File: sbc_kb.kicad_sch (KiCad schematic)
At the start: 18 parts, among them J1 Mini-DIN-6, J2 Mini-DIN-6, U4 7406, U9 VT82C42 PS2 CONTROLLER

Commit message: minor BOM tweaks due part availability. make some pcb routing a little nicer.
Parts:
- F1: LCSC Part # C3760254 -> C2687078
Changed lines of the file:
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@@
 			)
 		)
-		(property "Description" "LCSC #C3760254"
+		(property "Description" "LCSC #C3760254 (Bourns) or LCSC #C2687078"
 			(at 60.96 30.48 0)
 			(effects
@@
 			)
 		)
-		(property "LCSC Part #" "C3760254"
+		(property "LCSC Part #" "C2687078"
 			(at 60.96 30.48 0)
 			(effects

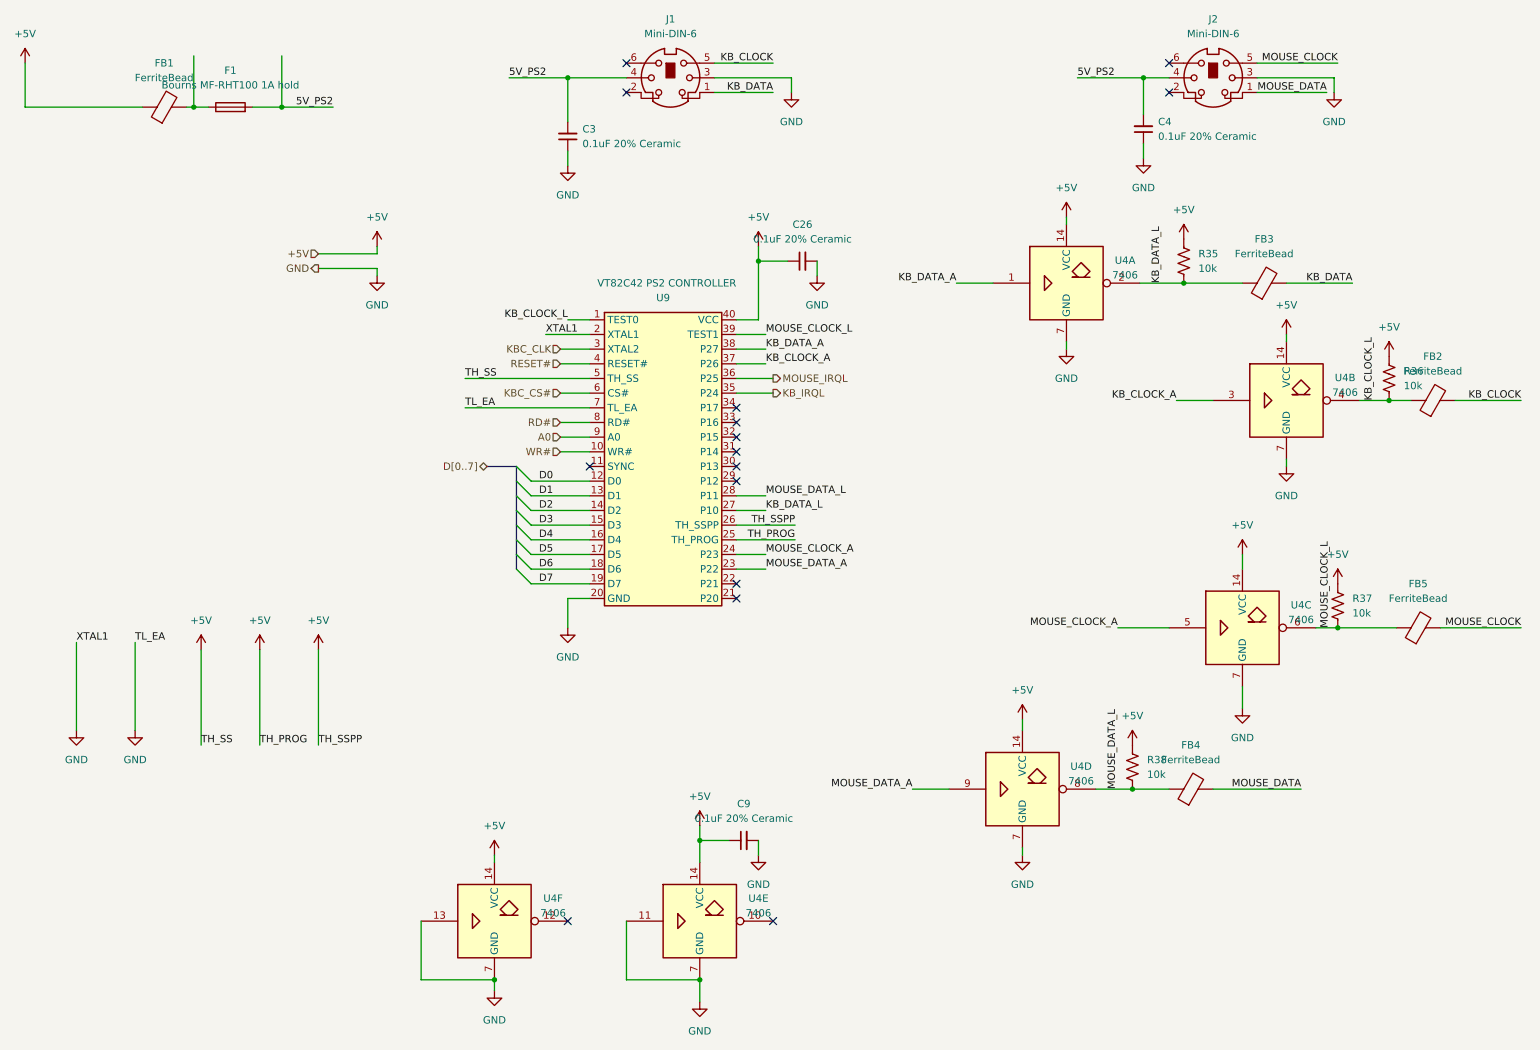
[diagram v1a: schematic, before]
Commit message: no more SMT for isa_i2c, tweak motherboard multiplex logic, handful of other tweaks
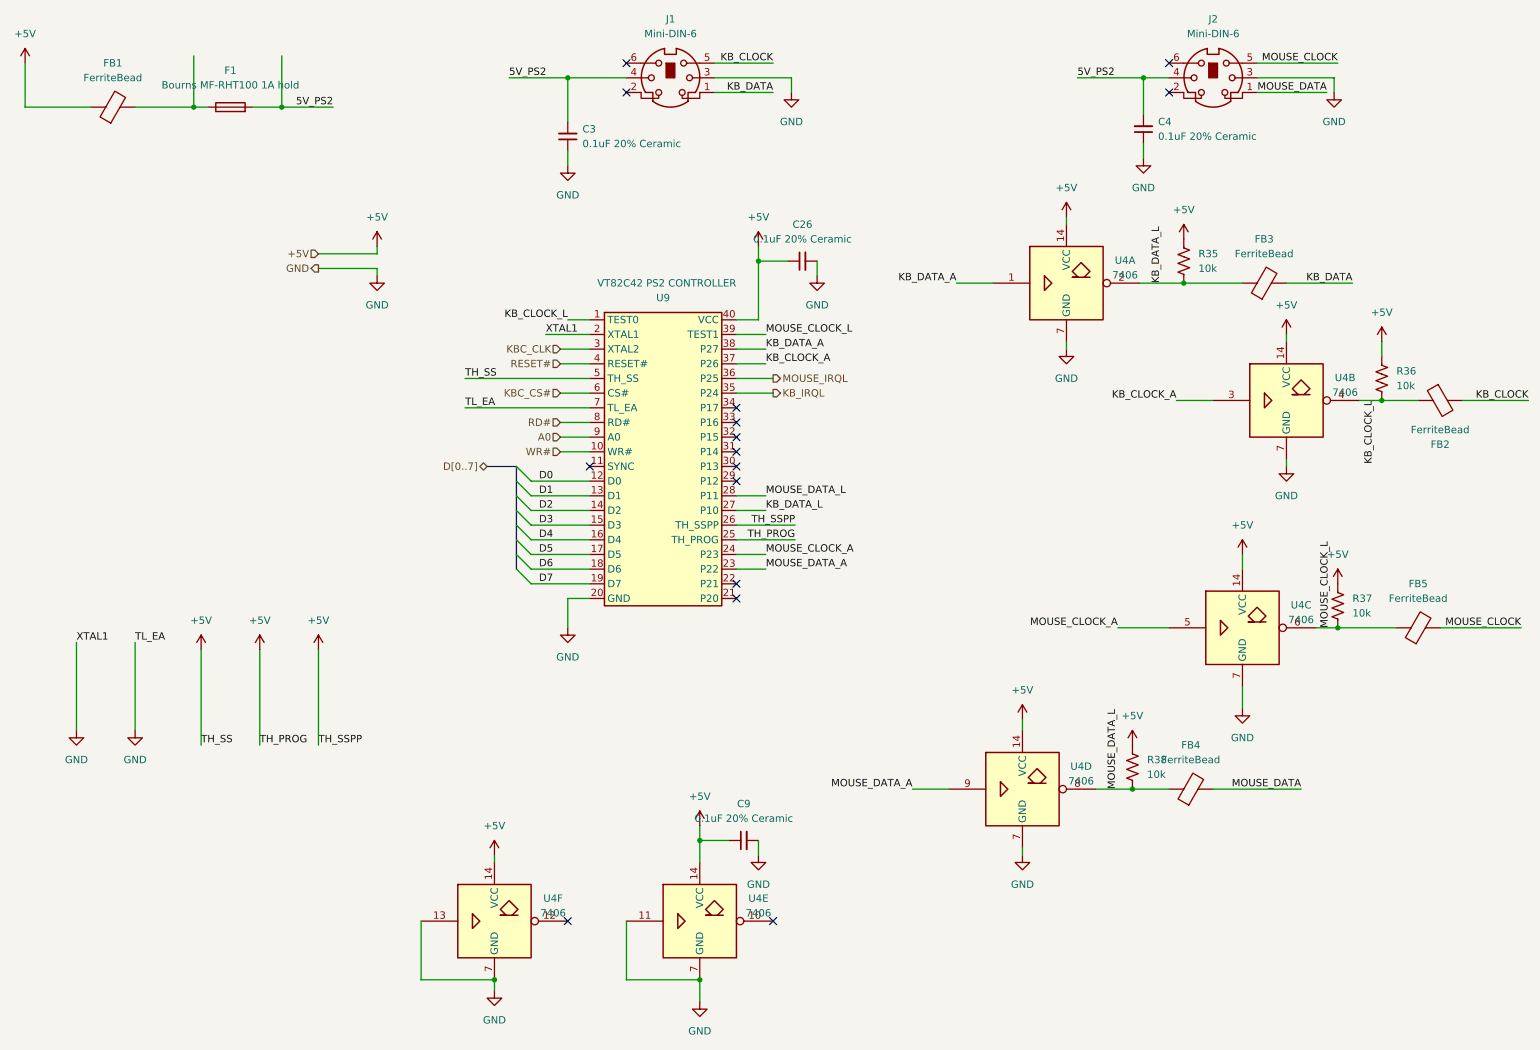
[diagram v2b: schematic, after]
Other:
- moved on the sheet: FB1, FB2, R36
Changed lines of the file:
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@@
 	)
 	(junction
+		(at 260.35 81.28)
+		(diameter 0)
+		(color 0 0 0 0)
+	)
+	(junction
 		(at 119.38 25.4)
 		(diameter 0)
@@
 		(color 0 0 0 0)
 	)
-	(junction
-		(at 261.62 81.28)
-		(diameter 0)
-		(color 0 0 0 0)
-	)
 	(no_connect
 		(at 129.54 27.94)
@@
 	(wire
 		(pts
-			(xy 25.4 30.48) (xy 45.72 30.48)
+			(xy 25.4 30.48) (xy 36.83 30.48)
 		)
 		(stroke
@@
 	(wire
 		(pts
-			(xy 53.34 30.48) (xy 54.61 30.48)
-		)
-		(stroke
-			(width 0)
-			(type default)
-		)
-	)
-	(wire
-		(pts
-			(xy 261.62 81.28) (xy 265.43 81.28)
+			(xy 44.45 30.48) (xy 54.61 30.48)
 		)
 		(stroke
@@
 	(wire
 		(pts
+			(xy 260.35 81.28) (xy 266.7 81.28)
+		)
+		(stroke
+			(width 0)
+			(type default)
+		)
+	)
+	(wire
+		(pts
 			(xy 231.14 148.59) (xy 246.38 148.59)
 		)
@@
 	(wire
 		(pts
-			(xy 256.54 81.28) (xy 261.62 81.28)
+			(xy 256.54 81.28) (xy 260.35 81.28)
 		)
 		(stroke
@@
 	(wire
 		(pts
+			(xy 260.35 73.66) (xy 260.35 71.12)
+		)
+		(stroke
+			(width 0)
+			(type default)
+		)
+	)
+	(wire
+		(pts
 			(xy 238.76 25.4) (xy 252.095 25.4)
 		)
@@
 	(wire
 		(pts
-			(xy 273.05 81.28) (xy 284.48 81.28)
+			(xy 274.32 81.28) (xy 285.75 81.28)
 		)
 		(stroke
@@
 	)
 	(label "KB_CLOCK"
-		(at 284.48 81.28 180)
+		(at 285.75 81.28 180)
 		(fields_autoplaced yes)
 		(effects
@@
 	)
 	(label "KB_CLOCK_L"
-		(at 259.08 81.28 90)
+		(at 259.08 81.28 270)
 		(fields_autoplaced yes)
 		(effects
@@
 				(size 1.27 1.27)
 			)
-			(justify left bottom)
+			(justify right bottom)
 		)
 	)
@@
 	(symbol
 		(lib_id "Device:FerriteBead")
-		(at 49.53 30.48 90)
+		(at 40.64 30.48 90)
 		(unit 1)
 		(exclude_from_sim no)
@@
 		(fields_autoplaced yes)
 		(property "Reference" "FB1"
-			(at 49.4792 22.86 90)
+			(at 40.5892 22.86 90)
 			(effects
 				(font
@@
 		)
 		(property "Value" "FerriteBead"
-			(at 49.4792 25.4 90)
+			(at 40.5892 25.4 90)
 			(effects
 				(font
@@
 		)
 		(property "Footprint" "Inductor_SMD:L_1206_3216Metric"
-			(at 49.53 32.258 90)
+			(at 40.64 32.258 90)
 			(effects
 				(font
@@
 		)
 		(property "Datasheet" "~"
-			(at 49.53 30.48 0)
+			(at 40.64 30.48 0)
 			(effects
 				(font
@@
 		)
 		(property "Description" "LCSC #C92887"
-			(at 49.53 30.48 0)
+			(at 40.64 30.48 0)
 			(effects
 				(font
@@
 		)
 		(property "Height" ""
-			(at 49.53 30.48 0)
+			(at 40.64 30.48 0)
 			(effects
 				(font
@@
 		)
 		(property "Manufacturer_Name" ""
-			(at 49.53 30.48 0)
+			(at 40.64 30.48 0)
 			(effects
 				(font
@@
 		)
 		(property "Manufacturer_Part_Number" ""
-			(at 49.53 30.48 0)
+			(at 40.64 30.48 0)
 			(effects
 				(font
@@
 		)
 		(property "Mouser Part Number" ""
-			(at 49.53 30.48 0)
+			(at 40.64 30.48 0)
 			(effects
 				(font
@@
 		)
 		(property "Mouser Price/Stock" ""
-			(at 49.53 30.48 0)
+			(at 40.64 30.48 0)
 			(effects
 				(font
@@
 		)
 		(property "LCSC Part #" "C92887"
-			(at 49.53 30.48 0)
+			(at 40.64 30.48 0)
 			(effects
 				(font
@@
 	(symbol
 		(lib_id "Device:R_US")
-		(at 261.62 77.47 0)
+		(at 260.35 77.47 0)
 		(unit 1)
 		(exclude_from_sim no)
@@
 		(fields_autoplaced yes)
 		(property "Reference" "R36"
-			(at 264.16 76.2 0)
+			(at 262.89 76.2 0)
 			(effects
 				(font
@@
 		)
 		(property "Value" "10k"
-			(at 264.16 78.74 0)
+			(at 262.89 78.74 0)
 			(effects
 				(font
@@
 		)
 		(property "Footprint" "Resistor_SMD:R_0805_2012Metric"
-			(at 262.636 77.724 90)
+			(at 261.366 77.724 90)
 			(effects
 				(font
@@
 		)
 		(property "Datasheet" "~"
-			(at 261.62 77.47 0)
+			(at 260.35 77.47 0)
 			(effects
 				(font
@@
 		)
 		(property "Description" "LCSC #C84376 "
-			(at 261.62 77.47 0)
+			(at 260.35 77.47 0)
 			(effects
 				(font
@@
 		)
 		(property "Height" ""
-			(at 261.62 77.47 0)
+			(at 260.35 77.47 0)
 			(effects
 				(font
@@
 		)
 		(property "Manufacturer_Name" ""
-			(at 261.62 77.47 0)
+			(at 260.35 77.47 0)
 			(effects
 				(font
@@
 		)
 		(property "Manufacturer_Part_Number" ""
-			(at 261.62 77.47 0)
+			(at 260.35 77.47 0)
 			(effects
 				(font
@@
 		)
 		(property "Mouser Part Number" ""
-			(at 261.62 77.47 0)
+			(at 260.35 77.47 0)
 			(effects
 				(font
@@
 		)
 		(property "Mouser Price/Stock" ""
-			(at 261.62 77.47 0)
+			(at 260.35 77.47 0)
 			(effects
 				(font
@@
 		)
 		(property "LCSC Part #" "C84376 "
-			(at 261.62 77.47 0)
+			(at 260.35 77.47 0)
 			(effects
 				(font
@@
 	(symbol
 		(lib_id "Device:FerriteBead")
-		(at 269.24 81.28 90)
+		(at 270.51 81.28 90)
+		(mirror x)
 		(unit 1)
 		(exclude_from_sim no)
@@
 		(dnp no)
 		(property "Reference" "FB2"
-			(at 269.1892 73.66 90)
+			(at 270.4592 88.9 90)
 			(effects
 				(font
@@
 		)
 		(property "Value" "FerriteBead"
-			(at 269.1892 76.2 90)
+			(at 270.4592 86.36 90)
 			(effects
 				(font
@@
 		)
 		(property "Footprint" "Inductor_SMD:L_1206_3216Metric"
-			(at 269.24 83.058 90)
+			(at 270.51 79.502 90)
 			(effects
 				(font
@@
 		)
 		(property "Datasheet" "~"
-			(at 269.24 81.28 0)
+			(at 270.51 81.28 0)
 			(effects
 				(font
@@
 		)
 		(property "Description" "LCSC #C92887"
-			(at 269.24 81.28 0)
+			(at 270.51 81.28 0)
 			(effects
 				(font
@@
 		)
 		(property "Height" ""
-			(at 269.24 81.28 0)
+			(at 270.51 81.28 0)
 			(effects
 				(font
@@
 		)
 		(property "Manufacturer_Name" ""
-			(at 269.24 81.28 0)
+			(at 270.51 81.28 0)
 			(effects
 				(font
@@
 		)
 		(property "Manufacturer_Part_Number" ""
-			(at 269.24 81.28 0)
+			(at 270.51 81.28 0)
 			(effects
 				(font
@@
 		)
 		(property "Mouser Part Number" ""
-			(at 269.24 81.28 0)
+			(at 270.51 81.28 0)
 			(effects
 				(font
@@
 		)
 		(property "Mouser Price/Stock" ""
-			(at 269.24 81.28 0)
+			(at 270.51 81.28 0)
 			(effects
 				(font
@@
 		)
 		(property "LCSC Part #" "C92887"
-			(at 269.24 81.28 0)
+			(at 270.51 81.28 0)
 			(effects
 				(font
@@
 	(symbol
 		(lib_id "power:+5V")
-		(at 261.62 73.66 0)
+		(at 260.35 71.12 0)
 		(unit 1)
 		(exclude_from_sim no)
@@
 		(fields_autoplaced yes)
 		(property "Reference" "#PWR0314"
-			(at 261.62 77.47 0)
+			(at 260.35 74.93 0)
 			(effects
 				(font
@@
 		)
 		(property "Value" "+5V"
-			(at 261.62 68.58 0)
+			(at 260.35 66.04 0)
 			(effects
 				(font
@@
 		)
 		(property "Footprint" ""
-			(at 261.62 73.66 0)
+			(at 260.35 71.12 0)
 			(effects
 				(font
@@
 		)
 		(property "Datasheet" ""
-			(at 261.62 73.66 0)
+			(at 260.35 71.12 0)
 			(effects
 				(font
@@
 		)
 		(property "Description" ""
-			(at 261.62 73.66 0)
+			(at 260.35 71.12 0)
 			(effects
 				(font

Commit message: motherboard tweaks for manufacturing run, i2c card tweaks for manufacturing run, de9 -> stemma adapter idea for the i2c card
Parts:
- C26, C3, C4, C9: LCSC Part # C1853649 -> C49678
- FB1, FB2, FB3, FB4, FB5: footprint Inductor_SMD:L_1206_3216Metric -> Inductor_SMD:L_0805_2012Metric; LCSC Part # C92887 -> C1015
- R35, R36, R37, R38: LCSC Part # C84376 -> C17414
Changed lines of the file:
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@@
 			)
 		)
-		(property "Footprint" "Inductor_SMD:L_1206_3216Metric"
+		(property "Footprint" "Inductor_SMD:L_0805_2012Metric"
 			(at 40.64 32.258 90)
 			(effects
@@
 			)
 		)
-		(property "Description" "LCSC #C92887"
+		(property "Description" "LCSC #C1015"
 			(at 40.64 30.48 0)
 			(effects
@@
 			)
 		)
-		(property "LCSC Part #" "C92887"
+		(property "LCSC Part #" "C1015"
 			(at 40.64 30.48 0)
 			(effects
@@
 			)
 		)
-		(property "Description" "LCSC #C84376"
+		(property "Description" "LCSC #C17414"
 			(at 260.35 77.47 0)
 			(effects
@@
 			)
 		)
-		(property "LCSC Part #" "C84376 "
+		(property "LCSC Part #" "C17414"
 			(at 260.35 77.47 0)
 			(effects
@@
 			)
 		)
-		(property "Description" "LCSC #C1853649"
+		(property "Description" "LCSC #C49678"
 			(at 119.38 35.56 0)
 			(effects
@@
 			)
 		)
-		(property "LCSC Part #" "C1853649"
+		(property "LCSC Part #" "C49678"
 			(at 119.38 35.56 0)
 			(effects
@@
 			)
 		)
-		(property "Description" "LCSC #C1853649"
+		(property "Description" "LCSC #C49678"
 			(at 160.02 57.15 0)
 			(effects
@@
 			)
 		)
-		(property "LCSC Part #" "C1853649"
+		(property "LCSC Part #" "C49678"
 			(at 160.02 57.15 0)
 			(effects
@@
 			)
 		)
-		(property "Description" "LCSC #C84376"
+		(property "Description" "LCSC #C17414"
 			(at 252.73 116.84 0)
 			(effects
@@
 			)
 		)
-		(property "LCSC Part #" "C84376 "
+		(property "LCSC Part #" "C17414"
 			(at 252.73 116.84 0)
 			(effects
@@
 			)
 		)
-		(property "Description" "LCSC #C84376"
+		(property "Description" "LCSC #C17414"
 			(at 226.06 57.15 0)
 			(effects
@@
 			)
 		)
-		(property "LCSC Part #" "C84376 "
+		(property "LCSC Part #" "C17414"
 			(at 226.06 57.15 0)
 			(effects
@@
 			)
 		)
-		(property "Description" "LCSC #C1853649"
+		(property "Description" "LCSC #C49678"
 			(at 149.86 157.48 0)
 			(effects
@@
 			)
 		)
-		(property "LCSC Part #" "C1853649"
+		(property "LCSC Part #" "C49678"
 			(at 149.86 157.48 0)
 			(effects
@@
 			)
 		)
-		(property "Footprint" "Inductor_SMD:L_1206_3216Metric"
+		(property "Footprint" "Inductor_SMD:L_0805_2012Metric"
 			(at 240.03 62.738 90)
 			(effects
@@
 			)
 		)
-		(property "Description" "LCSC #C92887"
+		(property "Description" "LCSC #C1015"
 			(at 240.03 60.96 0)
 			(effects
@@
 			)
 		)
-		(property "LCSC Part #" "C92887"
+		(property "LCSC Part #" "C1015"
 			(at 240.03 60.96 0)
 			(effects
@@
 			)
 		)
-		(property "Footprint" "Inductor_SMD:L_1206_3216Metric"
+		(property "Footprint" "Inductor_SMD:L_0805_2012Metric"
 			(at 270.51 79.502 90)
 			(effects
@@
 			)
 		)
-		(property "Description" "LCSC #C92887"
+		(property "Description" "LCSC #C1015"
 			(at 270.51 81.28 0)
 			(effects
@@
 			)
 		)
-		(property "LCSC Part #" "C92887"
+		(property "LCSC Part #" "C1015"
 			(at 270.51 81.28 0)
 			(effects
@@
 			)
 		)
-		(property "Description" "LCSC #C1853649"
+		(property "Description" "LCSC #C49678"
 			(at 219.075 34.29 0)
 			(effects
@@
 			)
 		)
-		(property "LCSC Part #" "C1853649"
+		(property "LCSC Part #" "C49678"
 			(at 219.075 34.29 0)
 			(effects
@@
 			)
 		)
-		(property "Footprint" "Inductor_SMD:L_1206_3216Metric"
+		(property "Footprint" "Inductor_SMD:L_0805_2012Metric"
 			(at 266.7 122.428 90)
 			(effects
@@
 			)
 		)
-		(property "Description" "LCSC #C92887"
+		(property "Description" "LCSC #C1015"
 			(at 266.7 120.65 0)
 			(effects
@@
 			)
 		)
-		(property "LCSC Part #" "C92887"
+		(property "LCSC Part #" "C1015"
 			(at 266.7 120.65 0)
 			(effects
@@
 			)
 		)
-		(property "Footprint" "Inductor_SMD:L_1206_3216Metric"
+		(property "Footprint" "Inductor_SMD:L_0805_2012Metric"
 			(at 227.33 150.368 90)
 			(effects
@@
 			)
 		)
-		(property "Description" "LCSC #C92887"
+		(property "Description" "LCSC #C1015"
 			(at 227.33 148.59 0)
 			(effects
@@
 			)
 		)
-		(property "LCSC Part #" "C92887"
+		(property "LCSC Part #" "C1015"
 			(at 227.33 148.59 0)
 			(effects
@@
 			)
 		)
-		(property "Description" "LCSC #C84376"
+		(property "Description" "LCSC #C17414"
 			(at 217.17 144.78 0)
 			(effects
@@
 			)
 		)
-		(property "LCSC Part #" "C84376 "
+		(property "LCSC Part #" "C17414"
 			(at 217.17 144.78 0)
 			(effects
